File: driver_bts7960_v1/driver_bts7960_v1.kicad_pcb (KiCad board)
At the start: 2 copper layers, 56.5 x 43.7 mm, 32 parts, among them J1 Motor_1, J2 Alimentacion, J3 Conn_02x04_Odd_Even, J6 Motor_2, U1 BTS7960B, U2 BTS7960B, U3 BTS7960B, U4 BTS7960B, U5 74HC244

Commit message: .
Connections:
- R4 pad 2: ENABLE_1 -> OUT_EN_1
- R5 pad 2: ENABLE_1 -> OUT_EN_1
- R7 pad 2: ENABLE_2 -> OUT_EN_2
- R9 pad 2: ENABLE_2 -> OUT_EN_2
- U5 pad 15: GND -> ENABLE_2
- U5 pad 17: GND -> ENABLE_1
- U5 pad 3: GND -> OUT_EN_1
- U5 pad 5: GND -> OUT_EN_2

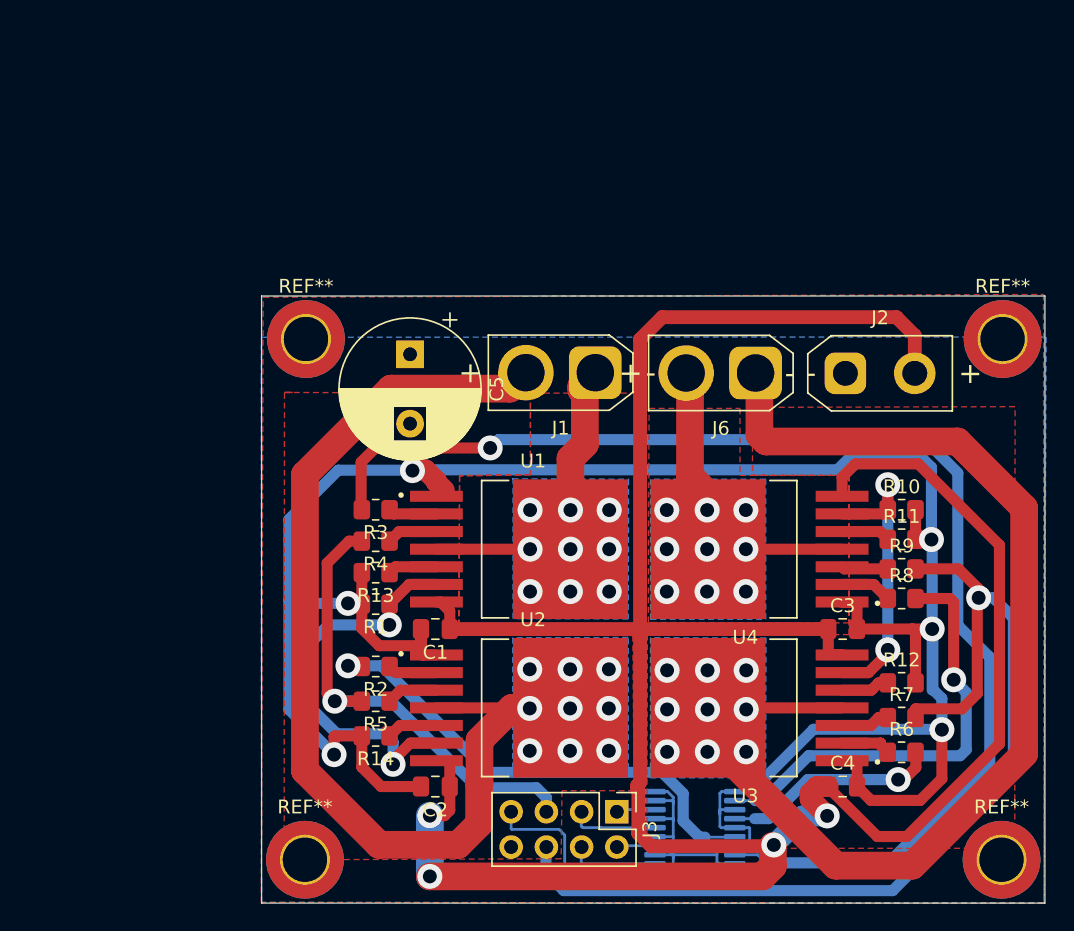
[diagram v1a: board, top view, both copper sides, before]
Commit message: .
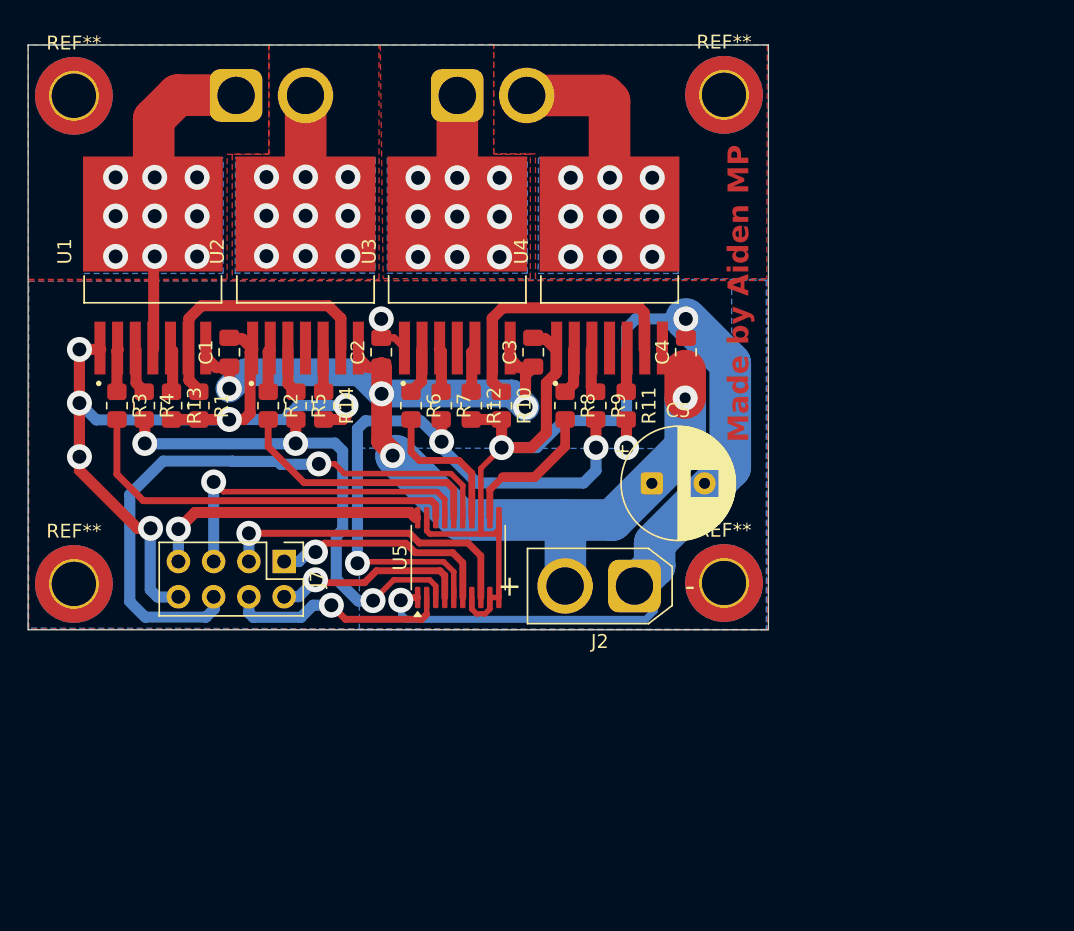
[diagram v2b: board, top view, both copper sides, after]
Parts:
- removed J3: Conn_02x04_Odd_Even, Connector_PinHeader_2.54mm:PinHeader_2x04_P2.54mm_Vertical
- removed the REF** at (178.8, 93.5)
- removed the REF** at (128.6, 56.0)
- removed the REF** at (178.8, 56.0)
- removed the REF** at (128.6, 93.5)
- added J7: Conn_02x04_Odd_Even, Connector_PinHeader_2.54mm:PinHeader_2x04_P2.54mm_Vertical, F.Cu at (127.1, 72.0)
- added REF**: MountingHole_3.2mm_M3_DIN965_Pad_TopBottom, MountingHole:MountingHole_3.2mm_M3_DIN965_Pad_TopBottom, F.Cu at (158.8, 38.4)
- added REF**: MountingHole_3.2mm_M3_DIN965_Pad_TopBottom, MountingHole:MountingHole_3.2mm_M3_DIN965_Pad_TopBottom, F.Cu at (111.9, 38.4)
- added REF**: MountingHole_3.2mm_M3_DIN965_Pad_TopBottom, MountingHole:MountingHole_3.2mm_M3_DIN965_Pad_TopBottom, F.Cu at (111.9, 73.6)
- added REF**: MountingHole_3.2mm_M3_DIN965_Pad_TopBottom, MountingHole:MountingHole_3.2mm_M3_DIN965_Pad_TopBottom, F.Cu at (158.8, 73.5)
- C5: footprint Capacitor_THT:CP_Radial_D10.0mm_P5.00mm -> Capacitor_THT:CP_Radial_D8.0mm_P3.80mm
- J1, J6: moved to B.Cu
- J2: value Alimentacion -> XT30; footprint Connector_AMASS:AMASS_XT30UPB-F_1x02_P5.0mm_Vertical -> Connector_AMASS:AMASS_XT30U-F_1x02_P5.0mm_Vertical
- U5: moved to F.Cu
- moved R6 43.3 mm to (136.2, 60.8), turned to -90 degrees
- moved R7 40.1 mm to (138.4, 60.8), turned to -90 degrees
- moved U3 38.6 mm to (139.5, 50.6), turned to 90 degrees
- moved R12 36.9 mm to (140.5, 60.8), turned to -90 degrees
- moved U2 35.4 mm to (128.6, 50.6), turned to 90 degrees
- moved U1 33.4 mm to (117.6, 50.6), turned to 90 degrees
- moved C4 33.3 mm to (156.0, 56.9), turned to 90 degrees
- moved J1 32.7 mm to (123.6, 38.4), turned to 0 degrees
- moved C2 31.5 mm to (134.1, 56.9), turned to 90 degrees
- moved C3 29.9 mm to (145.0, 56.9), turned to 90 degrees
- moved R10 29.8 mm to (142.7, 60.8), turned to -90 degrees
- moved J6 29.4 mm to (139.5, 38.4), turned to 0 degrees
- moved R8 28.0 mm to (147.3, 60.8), turned to -90 degrees
- moved U5 26.1 mm to (139.6, 71.7), turned to 90 degrees
- moved R9 25.0 mm to (149.5, 60.8), turned to -90 degrees
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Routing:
- net +24V: track 193.0 -> 79.9 mm, vias 4 -> 5
- net Net-(J6-Pin_1): track 85.3 -> 8.57 mm
- net Net-(J1-Pin_2): track 79.8 -> 8.66 mm
- net OUT_A: track 91.5 -> 28.7 mm, vias 1 -> 0
- net OUT_EN_2: track 0.00 -> 43.6 mm, vias 0 -> 3
- net OUT_EN_1: track 0.00 -> 37.5 mm, vias 0 -> 3
- net ENABLE_2: track 72.0 -> 43.5 mm
- net OUT_D: track 32.1 -> 10.7 mm, vias 1 -> 0
- net PWM_D: track 2.76 -> 21.7 mm, vias 0 -> 1
- net GND: track 198.1 -> 181.6 mm, vias 6 -> 11
- net OUT_B: track 35.1 -> 18.7 mm, vias 1 -> 0
- net PWM_B: track 2.74 -> 13.8 mm, vias 0 -> 1
- net PWM_C: track 6.30 -> 16.5 mm, vias 0 -> 1
- net ENABLE_1: track 34.4 -> 24.3 mm
- net PWM_A: track 6.51 -> 16.2 mm, vias 0 -> 1
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- added copper zone on B.Cu, net +24V
- added copper zone on F.Cu, net GND
- removed copper zone on F.Cu, net +24V
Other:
- board size 56.5 x 43.7 mm -> 53.4 x 42.1 mm
- board text added: "Made by Aiden MP"
